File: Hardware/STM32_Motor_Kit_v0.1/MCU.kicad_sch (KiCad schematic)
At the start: 17 parts, among them SW1 SW_DIP_x01, SW2 Push_Button_SMD_4P, U1 STM32G431RBT6, Y1 CRYSTAL_8mHz

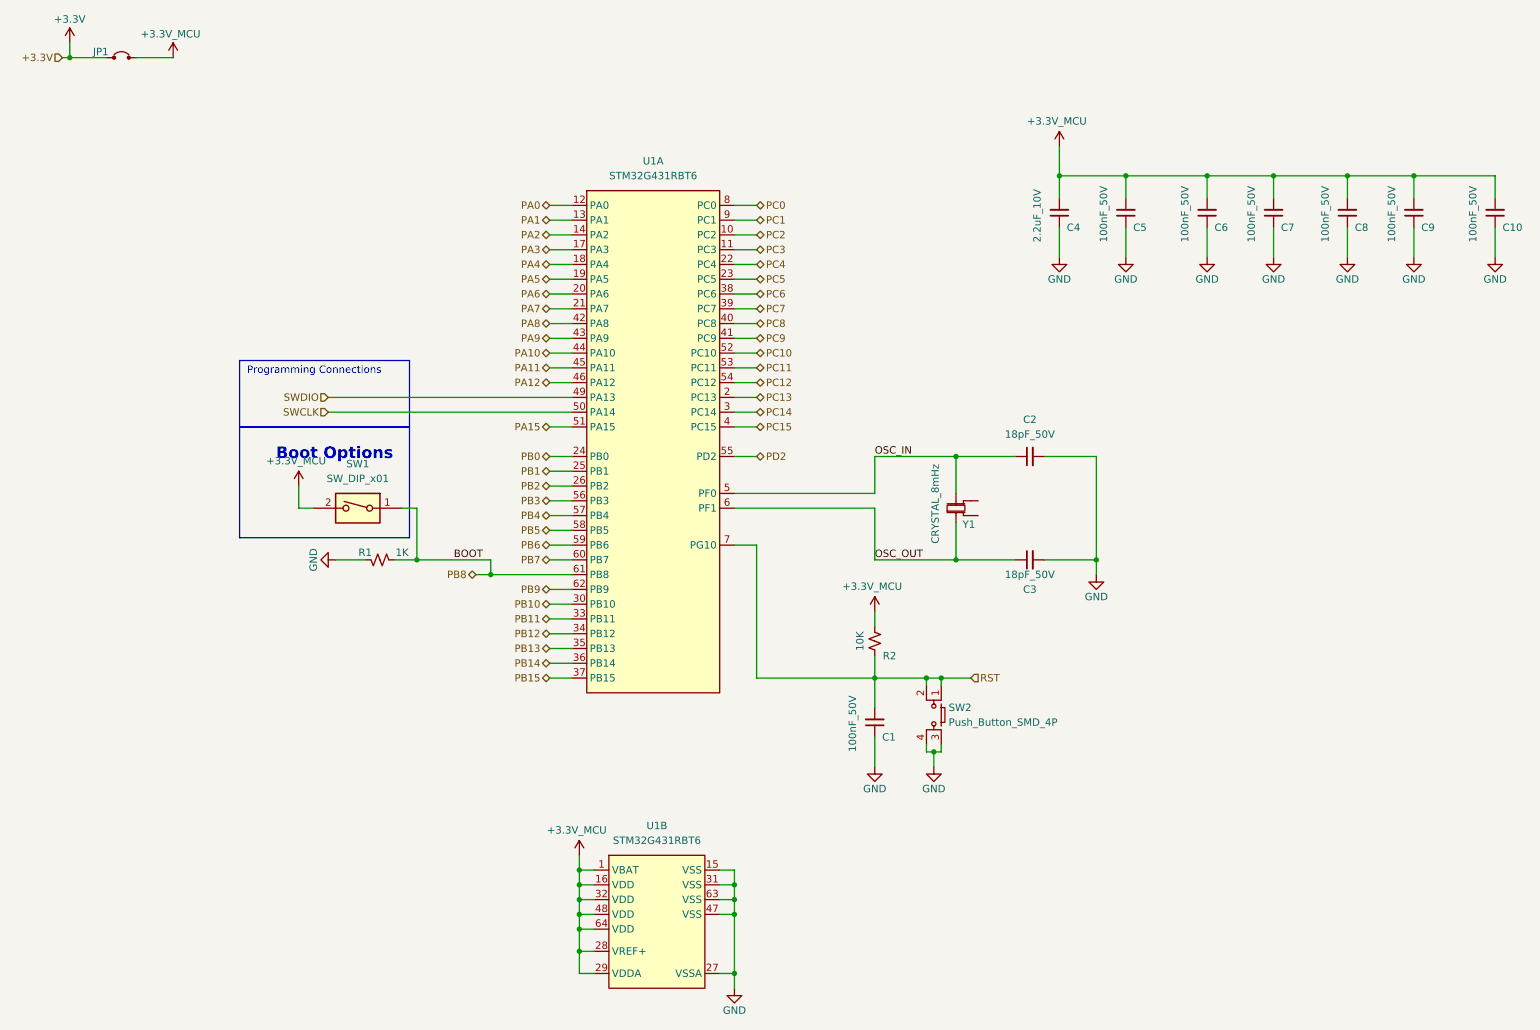
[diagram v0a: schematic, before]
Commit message: 12.01.2025
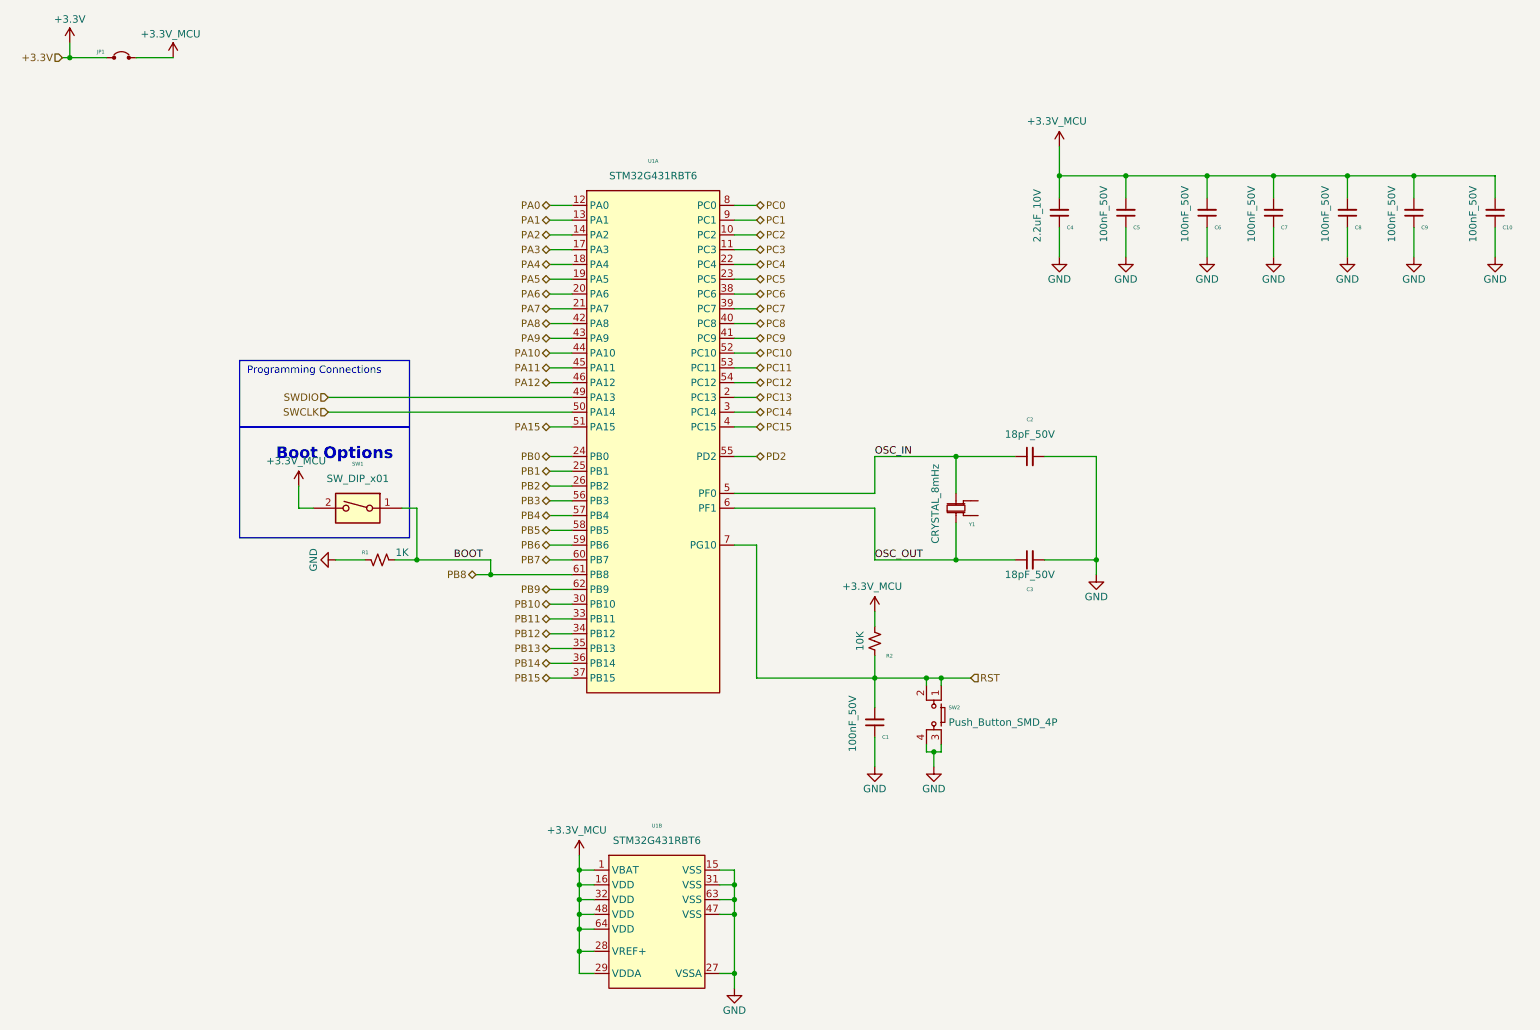
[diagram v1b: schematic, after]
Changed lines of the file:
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@@
 			(effects
 				(font
-					(size 1.27 1.27)
+					(face "Arial")
+					(size 0.635 0.635)
 				)
 				(hide yes)
@@
 			(effects
 				(font
-					(size 1.27 1.27)
+					(face "Arial")
+					(size 0.635 0.635)
 				)
 				(justify right)
@@
 			(effects
 				(font
-					(size 1.27 1.27)
+					(face "Arial")
+					(size 0.635 0.635)
 				)
 				(hide yes)
@@
 			(effects
 				(font
-					(size 1.27 1.27)
+					(face "Arial")
+					(size 0.635 0.635)
 				)
 				(hide yes)
@@
 			(effects
 				(font
-					(size 1.27 1.27)
+					(face "Arial")
+					(size 0.635 0.635)
 				)
 				(hide yes)
@@
 			(effects
 				(font
-					(size 1.27 1.27)
+					(face "Arial")
+					(size 0.635 0.635)
 				)
 			)
@@
 			(effects
 				(font
-					(size 1.27 1.27)
+					(face "Arial")
+					(size 0.635 0.635)
 				)
 				(justify right)
@@
 			(effects
 				(font
-					(size 1.27 1.27)
+					(face "Arial")
+					(size 0.635 0.635)
 				)
 				(hide yes)
@@
 			(effects
 				(font
-					(size 1.27 1.27)
+					(face "Arial")
+					(size 0.635 0.635)
 				)
 				(hide yes)
@@
 			(effects
 				(font
-					(size 1.27 1.27)
+					(face "Arial")
+					(size 0.635 0.635)
 				)
 				(hide yes)
@@
 			(effects
 				(font
-					(size 1.27 1.27)
+					(face "Arial")
+					(size 0.635 0.635)
 				)
 				(justify right)
@@
 			(effects
 				(font
-					(size 1.27 1.27)
+					(face "Arial")
+					(size 0.635 0.635)
 				)
 				(justify right)
@@
 			(effects
 				(font
-					(size 1.27 1.27)
+					(face "Arial")
+					(size 0.635 0.635)
 				)
 			)
@@
 			(effects
 				(font
-					(size 1.27 1.27)
+					(face "Arial")
+					(size 0.635 0.635)
 				)
 				(hide yes)
@@
 			(effects
 				(font
-					(size 1.27 1.27)
+					(face "Arial")
+					(size 0.635 0.635)
 				)
 				(hide yes)
@@
 			(effects
 				(font
-					(size 1.27 1.27)
+					(face "Arial")
+					(size 0.635 0.635)
 				)
 			)
@@
 			(effects
 				(font
-					(size 1.27 1.27)
+					(face "Arial")
+					(size 0.635 0.635)
 				)
 			)
@@
 			(effects
 				(font
-					(size 1.27 1.27)
+					(face "Arial")
+					(size 0.635 0.635)
 				)
 			)
@@
 			(effects
 				(font
-					(size 1.27 1.27)
+					(face "Arial")
+					(size 0.635 0.635)
 				)
 				(hide yes)
@@
 			(effects
 				(font
-					(size 1.27 1.27)
+					(face "Arial")
+					(size 0.635 0.635)
 				)
 				(hide yes)
@@
 			(effects
 				(font
-					(size 1.27 1.27)
+					(face "Arial")
+					(size 0.635 0.635)
 				)
 			)
@@
 			(effects
 				(font
-					(size 1.27 1.27)
+					(face "Arial")
+					(size 0.635 0.635)
 				)
 				(justify right)
@@
 			(effects
 				(font
-					(size 1.27 1.27)
+					(face "Arial")
+					(size 0.635 0.635)
 				)
 				(justify right)
@@
 			(effects
 				(font
-					(size 1.27 1.27)
+					(face "Arial")
+					(size 0.635 0.635)
 				)
 				(hide yes)
@@
 			(effects
 				(font
-					(size 1.27 1.27)
+					(face "Arial")
+					(size 0.635 0.635)
 				)
 				(hide yes)
@@
 			(effects
 				(font
-					(size 1.27 1.27)
+					(face "Arial")
+					(size 0.635 0.635)
 				)
 				(justify right)
@@
 			(effects
 				(font
-					(size 1.27 1.27)
+					(face "Arial")
+					(size 0.635 0.635)
 				)
 			)
@@
 			(effects
 				(font
-					(size 1.27 1.27)
+					(face "Arial")
+					(size 0.635 0.635)
 				)
 			)
@@
 			(effects
 				(font
-					(size 1.27 1.27)
+					(face "Arial")
+					(size 0.635 0.635)
 				)
 				(hide yes)
@@
 			(effects
 				(font
-					(size 1.27 1.27)
+					(face "Arial")
+					(size 0.635 0.635)
 				)
 				(justify right)
@@
 			(effects
 				(font
-					(size 1.27 1.27)
+					(face "Arial")
+					(size 0.635 0.635)
 				)
 				(justify right)
@@
 			(effects
 				(font
-					(size 1.27 1.27)
+					(face "Arial")
+					(size 0.635 0.635)
 				)
 				(hide yes)
@@
 			(effects
 				(font
-					(size 1.27 1.27)
+					(face "Arial")
+					(size 0.635 0.635)
 				)
 				(hide yes)
@@
 			(effects
 				(font
-					(size 1.27 1.27)
+					(face "Arial")
+					(size 0.635 0.635)
 				)
 				(hide yes)
@@
 			(effects
 				(font
-					(size 1.27 1.27)
+					(face "Arial")
+					(size 0.635 0.635)
 				)
 				(justify left)
@@
 			(effects
 				(font
-					(size 1.27 1.27)
-				)
-				(hide yes)
+					(face "Arial")
+					(size 0.635 0.635)
+				)
+				(hide yes)
